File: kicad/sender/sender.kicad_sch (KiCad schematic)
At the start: 18 parts, among them J1 RJ45, J2 Screw_Terminal_01x03, J3 Conn_01x10_Pin, J4 Conn_01x08_Pin, J5 Conn_01x06_Pin, J6 Conn_01x08_Pin, Q1 IRLZ44N, Q2 IRLZ44N, Q3 IRLZ44N, U1 MAX481E, U2 6N137

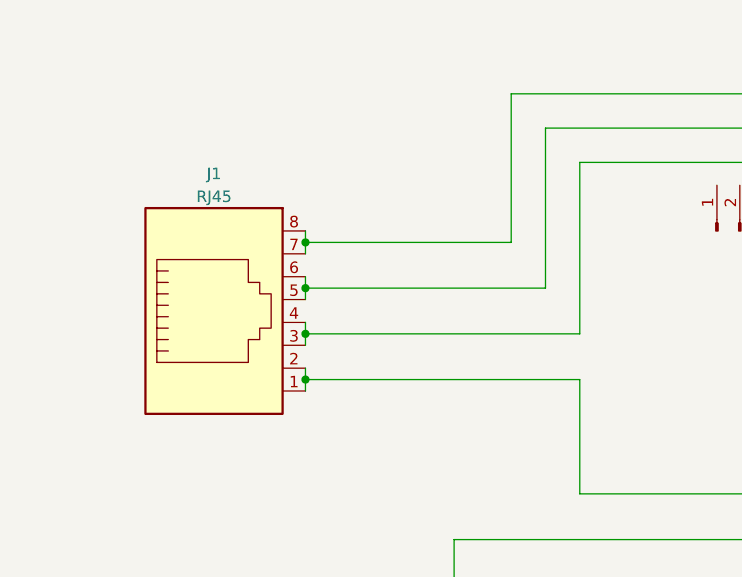
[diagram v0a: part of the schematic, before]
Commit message: Add files via upload
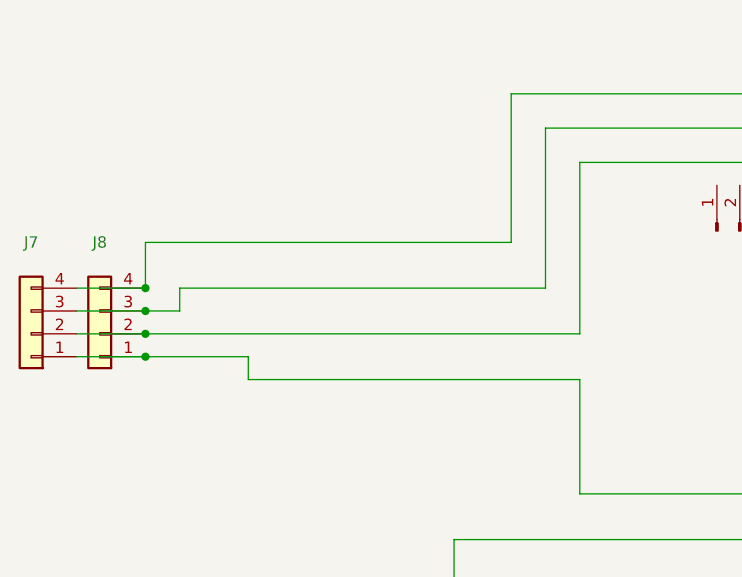
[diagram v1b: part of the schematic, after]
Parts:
- removed J1: RJ45, Connector_RJ:RJ45_Amphenol_54602-x08_Horizontal, symbol Connector:RJ45
- added J7, J8: Conn_01x04, Connector_PinHeader_2.00mm:PinHeader_1x04_P2.00mm_Vertical, symbol Connector_Generic:Conn_01x04
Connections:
- net at C1.1, C2.2, J2.1 (Pin_1)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: now also J7.1 (Pin_1), J8.1 (Pin_1)
- net at Q1.2 (D): now also J7.2 (Pin_2), J8.2 (Pin_2)
- net at Q2.2 (D): now also J7.3 (Pin_3), J8.3 (Pin_3)
- net at Q3.2 (D): now also J7.4 (Pin_4), J8.4 (Pin_4)
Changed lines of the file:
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@@
   (junction (at 151.13 133.35) (diameter 0) (color 0 0 0 0)
   )
+  (junction (at 45.72 87.63) (diameter 0) (color 0 0 0 0)
+  )
   (junction (at 165.1 148.59) (diameter 0) (color 0 0 0 0)
   )
   (junction (at 182.88 148.59) (diameter 0) (color 0 0 0 0)
   )
+  (junction (at 45.72 82.55) (diameter 0) (color 0 0 0 0)
+  )
   (junction (at 157.48 50.8) (diameter 0) (color 0 0 0 0)
   )
-  (junction (at 63.5 82.55) (diameter 0) (color 0 0 0 0)
-  )
   (junction (at 96.52 121.92) (diameter 0) (color 0 0 0 0)
   )
-  (junction (at 63.5 77.47) (diameter 0) (color 0 0 0 0)
-  )
   (junction (at 115.57 105.41) (diameter 0) (color 0 0 0 0)
   )
@@
   (junction (at 151.13 130.81) (diameter 0) (color 0 0 0 0)
   )
-  (junction (at 63.5 87.63) (diameter 0) (color 0 0 0 0)
-  )
   (junction (at 133.35 101.6) (diameter 0) (color 0 0 0 0)
   )
@@
   (junction (at 96.52 130.81) (diameter 0) (color 0 0 0 0)
   )
+  (junction (at 45.72 90.17) (diameter 0) (color 0 0 0 0)
+  )
   (junction (at 151.13 105.41) (diameter 0) (color 0 0 0 0)
   )
+  (junction (at 45.72 85.09) (diameter 0) (color 0 0 0 0)
+  )
   (junction (at 203.2 50.8) (diameter 0) (color 0 0 0 0)
   )
@@
   (junction (at 133.35 105.41) (diameter 0) (color 0 0 0 0)
   )
-  (junction (at 63.5 92.71) (diameter 0) (color 0 0 0 0)
-  )
-  (wire (pts (xy 63.5 87.63) (xy 93.98 87.63))
-    (stroke (width 0) (type default))
-  )
-  (wire (pts (xy 63.5 81.28) (xy 63.5 82.55))
+  (wire (pts (xy 45.72 87.63) (xy 93.98 87.63))
     (stroke (width 0) (type default))
   )
@@
     (stroke (width 0) (type default))
   )
-  (wire (pts (xy 63.5 86.36) (xy 63.5 87.63))
-    (stroke (width 0) (type default))
-  )
   (wire (pts (xy 142.24 128.27) (xy 137.16 128.27))
     (stroke (width 0) (type default))
@@
     (stroke (width 0) (type default))
   )
+  (wire (pts (xy 45.72 77.47) (xy 45.72 82.55))
+    (stroke (width 0) (type default))
+  )
   (wire (pts (xy 151.13 133.35) (xy 154.94 133.35))
     (stroke (width 0) (type default))
@@
     (stroke (width 0) (type default))
   )
+  (wire (pts (xy 45.72 85.09) (xy 49.53 85.09))
+    (stroke (width 0) (type default))
+  )
   (wire (pts (xy 80.01 110.49) (xy 80.01 119.38))
     (stroke (width 0) (type default))
   )
+  (wire (pts (xy 49.53 82.55) (xy 90.17 82.55))
+    (stroke (width 0) (type default))
+  )
   (wire (pts (xy 140.97 57.15) (xy 208.28 57.15))
     (stroke (width 0) (type default))
@@
     (stroke (width 0) (type default))
   )
-  (wire (pts (xy 63.5 91.44) (xy 63.5 92.71))
-    (stroke (width 0) (type default))
-  )
   (wire (pts (xy 129.54 45.72) (xy 129.54 71.12))
     (stroke (width 0) (type default))
   )
+  (wire (pts (xy 49.53 82.55) (xy 49.53 85.09))
+    (stroke (width 0) (type default))
+  )
   (wire (pts (xy 226.06 30.48) (xy 226.06 40.64))
     (stroke (width 0) (type default))
   )
-  (wire (pts (xy 63.5 92.71) (xy 63.5 93.98))
+  (wire (pts (xy 38.1 87.63) (xy 45.72 87.63))
     (stroke (width 0) (type default))
   )
@@
     (stroke (width 0) (type default))
   )
-  (wire (pts (xy 63.5 82.55) (xy 63.5 83.82))
+  (wire (pts (xy 38.1 90.17) (xy 45.72 90.17))
     (stroke (width 0) (type default))
   )
@@
     (stroke (width 0) (type default))
   )
-  (wire (pts (xy 63.5 76.2) (xy 63.5 77.47))
+  (wire (pts (xy 57.15 90.17) (xy 57.15 92.71))
     (stroke (width 0) (type default))
   )
@@
     (stroke (width 0) (type default))
   )
-  (wire (pts (xy 63.5 77.47) (xy 86.36 77.47))
-    (stroke (width 0) (type default))
-  )
   (wire (pts (xy 151.13 133.35) (xy 151.13 148.59))
     (stroke (width 0) (type default))
@@
     (stroke (width 0) (type default))
   )
+  (wire (pts (xy 45.72 77.47) (xy 86.36 77.47))
+    (stroke (width 0) (type default))
+  )
   (wire (pts (xy 165.1 148.59) (xy 151.13 148.59))
     (stroke (width 0) (type default))
   )
-  (wire (pts (xy 63.5 92.71) (xy 93.98 92.71))
+  (wire (pts (xy 57.15 92.71) (xy 93.98 92.71))
     (stroke (width 0) (type default))
   )
@@
     (stroke (width 0) (type default))
   )
+  (wire (pts (xy 38.1 85.09) (xy 45.72 85.09))
+    (stroke (width 0) (type default))
+  )
   (wire (pts (xy 86.36 60.96) (xy 143.51 60.96))
     (stroke (width 0) (type default))
@@
     (stroke (width 0) (type default))
   )
+  (wire (pts (xy 45.72 90.17) (xy 57.15 90.17))
+    (stroke (width 0) (type default))
+  )
   (wire (pts (xy 93.98 87.63) (xy 93.98 68.58))
     (stroke (width 0) (type default))
   )
+  (wire (pts (xy 38.1 82.55) (xy 45.72 82.55))
+    (stroke (width 0) (type default))
+  )
   (wire (pts (xy 90.17 64.77) (xy 90.17 82.55))
     (stroke (width 0) (type default))
@@
     (stroke (width 0) (type default))
   )
-  (wire (pts (xy 63.5 77.47) (xy 63.5 78.74))
-    (stroke (width 0) (type default))
-  )
   (wire (pts (xy 203.2 34.29) (xy 147.32 34.29))
     (stroke (width 0) (type default))
@@
     (stroke (width 0) (type default))
   )
-  (wire (pts (xy 63.5 87.63) (xy 63.5 88.9))
-    (stroke (width 0) (type default))
-  )
   (wire (pts (xy 151.13 105.41) (xy 157.48 105.41))
     (stroke (width 0) (type default))
@@
   )
   (wire (pts (xy 175.26 135.89) (xy 180.34 135.89))
-    (stroke (width 0) (type default))
-  )
-  (wire (pts (xy 90.17 82.55) (xy 63.5 82.55))
     (stroke (width 0) (type default))
   )
@@
     )
   )
-  (symbol (lib_id "Connector:RJ45") (at 53.34 86.36 0) (unit 1)
-    (in_bom yes) (on_board yes) (dnp no) (fields_autoplaced)
-    (property "Reference" "J1" (at 53.34 69.85 0)
-      (effects (font (size 1.27 1.27)))
-    )
-    (property "Value" "RJ45" (at 53.34 72.39 0)
-      (effects (font (size 1.27 1.27)))
-    )
-    (property "Footprint" "Connector_RJ:RJ45_Amphenol_54602-x08_Horizontal" (at 53.34 85.725 90)
-      (effects (font (size 1.27 1.27)) hide)
-    )
-    (property "Datasheet" "~" (at 53.34 85.725 90)
-      (effects (font (size 1.27 1.27)) hide)
-    )
-    (pin "1")
-    (pin "2")
-    (pin "3")
-    (pin "4")
-    (pin "5")
-    (pin "6")
-    (pin "7")
-    (pin "8")
-    (instances
-      (project "sender"
-        (path "/1a0e8450-7cd1-48c4-a620-76bc1dbc1086"
-          (reference "J1") (unit 1)
-        )
-      )
-    )
-  )
   (symbol (lib_id "Device:R") (at 146.05 128.27 90) (unit 1)
     (in_bom yes) (on_board yes) (dnp no) (fields_autoplaced)
@@
         )
       )
+    )
+  )
+  (symbol (lib_id "Connector_Generic:Conn_01x04") (at 40.64 87.63 180) (unit 1)
+    (in_bom yes) (on_board yes) (dnp no) (fields_autoplaced)
+    (property "Reference" "J8" (at 40.64 77.47 0)
+      (effects (font (size 1.27 1.27)))
+    )
+    (property "Value" "Conn_01x04" (at 40.64 80.01 0)
+      (effects (font (size 1.27 1.27)) hide)
+    )
+    (property "Footprint" "Connector_PinHeader_2.00mm:PinHeader_1x04_P2.00mm_Vertical" (at 40.64 87.63 0)
+      (effects (font (size 1.27 1.27)) hide)
+    )
+    (property "Datasheet" "~" (at 40.64 87.63 0)
+      (effects (font (size 1.27 1.27)) hide)
+    )
+    (pin "1")
+    (pin "2")
+    (pin "3")
+    (pin "4")
+    (instances
+      (project "sender"
+        (path "/1a0e8450-7cd1-48c4-a620-76bc1dbc1086"
+          (reference "J8") (unit 1)
+        )
+      )
+    )
+  )
+  (symbol (lib_id "Connector_Generic:Conn_01x04") (at 33.02 87.63 180) (unit 1)
+    (in_bom yes) (on_board yes) (dnp no) (fields_autoplaced)
+    (property "Reference" "J7" (at 33.02 77.47 0)
+      (effects (font (size 1.27 1.27)))
+    )
+    (property "Value" "Conn_01x04" (at 33.02 80.01 0)
+      (effects (font (size 1.27 1.27)) hide)
+    )
+    (property "Footprint" "Connector_PinHeader_2.00mm:PinHeader_1x04_P2.00mm_Vertical" (at 33.02 87.63 0)
+      (effects (font (size 1.27 1.27)) hide)
+    )
+    (property "Datasheet" "~" (at 33.02 87.63 0)
+      (effects (font (size 1.27 1.27)) hide)
+    )
+    (pin "1")
+    (pin "2")
+    (pin "3")
+    (pin "4")
+    (instances
+      (project "sender"
+        (path "/1a0e8450-7cd1-48c4-a620-76bc1dbc1086"
+          (reference "J7") (unit 1)
+        )
+      )
